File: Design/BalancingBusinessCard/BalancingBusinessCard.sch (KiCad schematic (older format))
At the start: 8 parts, among them J101 TestPoints, U101 ATtiny261-20SU

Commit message: Footprint assignment
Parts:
- C101, C102: footprint (none) -> Capacitor_SMD:C_0805_2012Metric
- R101, R102: footprint (none) -> Resistor_SMD:R_0603_1608Metric
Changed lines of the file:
@@
 F 0 "R102" H 7420 1196 50  0000 L CNN
 F 1 "1k" H 7420 1105 50  0000 L CNN
-F 2 "" V 7280 1150 50  0001 C CNN
+F 2 "Resistor_SMD:R_0603_1608Metric" V 7280 1150 50  0001 C CNN
 F 3 "~" H 7350 1150 50  0001 C CNN
 	1    7350 1150
@@
 F 0 "R101" H 6950 1350 50  0000 L CNN
 F 1 "1k" H 6950 1250 50  0000 L CNN
-F 2 "" V 7030 1250 50  0001 C CNN
+F 2 "Resistor_SMD:R_0603_1608Metric" V 7030 1250 50  0001 C CNN
 F 3 "~" H 7100 1250 50  0001 C CNN
 	1    7100 1250
@@
 F 0 "C102" H 5265 1296 50  0000 L CNN
 F 1 "10uF" H 5265 1205 50  0000 L CNN
-F 2 "" H 5188 1100 50  0001 C CNN
+F 2 "Capacitor_SMD:C_0805_2012Metric" H 5188 1100 50  0001 C CNN
 F 3 "~" H 5150 1250 50  0001 C CNN
 	1    5150 1250
@@
 F 0 "C101" V 3852 2400 50  0000 C CNN
 F 1 "10uF" V 3761 2400 50  0000 C CNN
-F 2 "" H 3638 2250 50  0001 C CNN
+F 2 "Capacitor_SMD:C_0805_2012Metric" H 3638 2250 50  0001 C CNN
 F 3 "~" H 3600 2400 50  0001 C CNN
 	1    3600 2400

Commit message: Added regulator
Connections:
- wire segments 17 -> 21
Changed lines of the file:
@@
 $Descr A4 11693 8268
 encoding utf-8
-Sheet 1 4
+Sheet 1 5
 Title ""
 Date ""
@@
 Text Label 5450 6050 1    50   ~ 0
 LED_3
+$Comp
+L power:PWR_FLAG #FLG0101
+U 1 1 5BCC0D87
+P 4050 1100
+F 0 "#FLG0101" H 4050 1175 50  0001 C CNN
+F 1 "PWR_FLAG" H 4050 1274 50  0000 C CNN
+F 2 "" H 4050 1100 50  0001 C CNN
+F 3 "~" H 4050 1100 50  0001 C CNN
+	1    4050 1100
+	1    0    0    -1
+$EndComp
+Wire Wire Line
+	4050 1100 4400 1100
+$Comp
+L power:PWR_FLAG #FLG0102
+U 1 1 5BCC114E
+P 4050 1400
+F 0 "#FLG0102" H 4050 1475 50  0001 C CNN
+F 1 "PWR_FLAG" H 4050 1574 50  0000 C CNN
+F 2 "" H 4050 1400 50  0001 C CNN
+F 3 "~" H 4050 1400 50  0001 C CNN
+	1    4050 1400
+	1    0    0    -1
+$EndComp
+Wire Wire Line
+	4050 1450 4050 1400
+$Comp
+L power:GND #PWR0134
+U 1 1 5BCC13FA
+P 4050 1450
+F 0 "#PWR0134" H 4050 1200 50  0001 C CNN
+F 1 "GND" H 4055 1277 50  0000 C CNN
+F 2 "" H 4050 1450 50  0001 C CNN
+F 3 "" H 4050 1450 50  0001 C CNN
+	1    4050 1450
+	1    0    0    -1
+$EndComp
+$Sheet
+S 1050 800  1350 350
+U 5BCC40AE
+F0 "1v8 Regulator" 50
+F1 "ft550.sch" 50
+F2 "Vin" I R 2400 900 50
+F3 "Vout" I R 2400 1000 50
+$EndSheet
+$Comp
+L power:+BATT #PWR?
+U 1 1 5BCC563A
+P 2500 900
+F 0 "#PWR?" H 2500 750 50  0001 C CNN
+F 1 "+BATT" H 2515 1073 50  0000 C CNN
+F 2 "" H 2500 900 50  0001 C CNN
+F 3 "" H 2500 900 50  0001 C CNN
+	1    2500 900
+	1    0    0    -1
+$EndComp
+Wire Wire Line
+	2500 900  2400 900
+$Comp
+L power:+1V8 #PWR?
+U 1 1 5BCC5911
+P 2650 1000
+F 0 "#PWR?" H 2650 850 50  0001 C CNN
+F 1 "+1V8" H 2665 1173 50  0000 C CNN
+F 2 "" H 2650 1000 50  0001 C CNN
+F 3 "" H 2650 1000 50  0001 C CNN
+	1    2650 1000
+	1    0    0    -1
+$EndComp
+Wire Wire Line
+	2650 1000 2400 1000
 $EndSCHEMATC

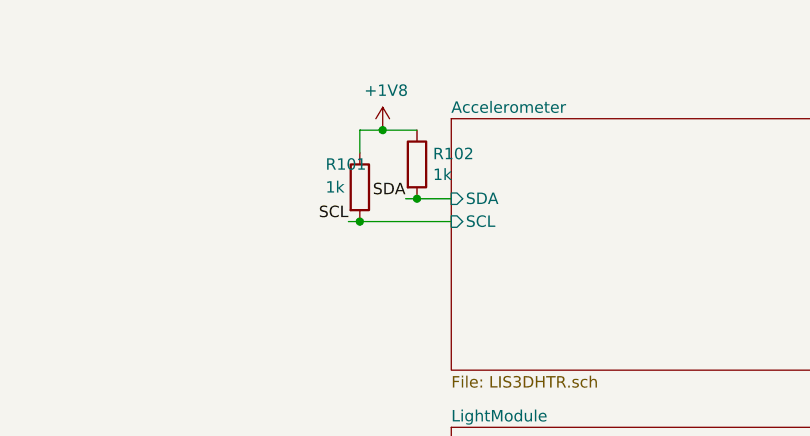
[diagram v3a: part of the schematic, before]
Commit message: Programming starting
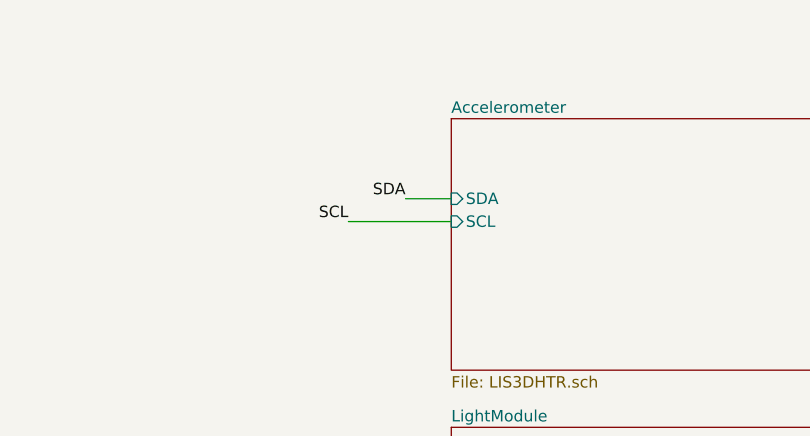
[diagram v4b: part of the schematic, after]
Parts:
- removed R101, R102: 1k, Resistor_SMD:R_0603_1608Metric, symbol Device:R
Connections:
- wire segments 21 -> 16
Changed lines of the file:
@@
 Text Label 7050 1400 2    50   ~ 0
 SCL
-Wire Wire Line
-	7500 1300 7350 1300
-$Comp
-L Device:R R102
-U 1 1 5BCC12E2
-P 7350 1150
-F 0 "R102" H 7420 1196 50  0000 L CNN
-F 1 "1k" H 7420 1105 50  0000 L CNN
-F 2 "Resistor_SMD:R_0603_1608Metric" V 7280 1150 50  0001 C CNN
-F 3 "~" H 7350 1150 50  0001 C CNN
-	1    7350 1150
-	1    0    0    -1
-$EndComp
-Wire Wire Line
-	7300 1300 7350 1300
-Connection ~ 7350 1300
-$Comp
-L power:+1V8 #PWR0110
-U 1 1 5BCC13E8
-P 7200 1000
-F 0 "#PWR0110" H 7200 850 50  0001 C CNN
-F 1 "+1V8" H 7215 1173 50  0000 C CNN
-F 2 "" H 7200 1000 50  0001 C CNN
-F 3 "" H 7200 1000 50  0001 C CNN
-	1    7200 1000
-	1    0    0    -1
-$EndComp
-Wire Wire Line
-	7350 1000 7200 1000
-Wire Wire Line
-	7200 1000 7100 1000
-Connection ~ 7200 1000
-$Comp
-L Device:R R101
-U 1 1 5BCC14CF
-P 7100 1250
-F 0 "R101" H 6950 1350 50  0000 L CNN
-F 1 "1k" H 6950 1250 50  0000 L CNN
-F 2 "Resistor_SMD:R_0603_1608Metric" V 7030 1250 50  0001 C CNN
-F 3 "~" H 7100 1250 50  0001 C CNN
-	1    7100 1250
-	1    0    0    -1
-$EndComp
-Wire Wire Line
-	7100 1000 7100 1100
-Wire Wire Line
-	7050 1400 7100 1400
-Wire Wire Line
-	7100 1400 7500 1400
-Connection ~ 7100 1400
 Text Label 7500 3800 2    50   ~ 0
 ADC0
@@
 Wire Wire Line
 	2650 1000 2400 1000
+Wire Wire Line
+	7300 1300 7500 1300
+Wire Wire Line
+	7050 1400 7500 1400
 $EndSCHEMATC
